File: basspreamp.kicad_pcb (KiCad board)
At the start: 2 copper layers, 62.2 x 44.5 mm, 27 parts, among them P1 INPUT, P2 OUTPUT, P3 Power, Q1 J201, U1 TL072

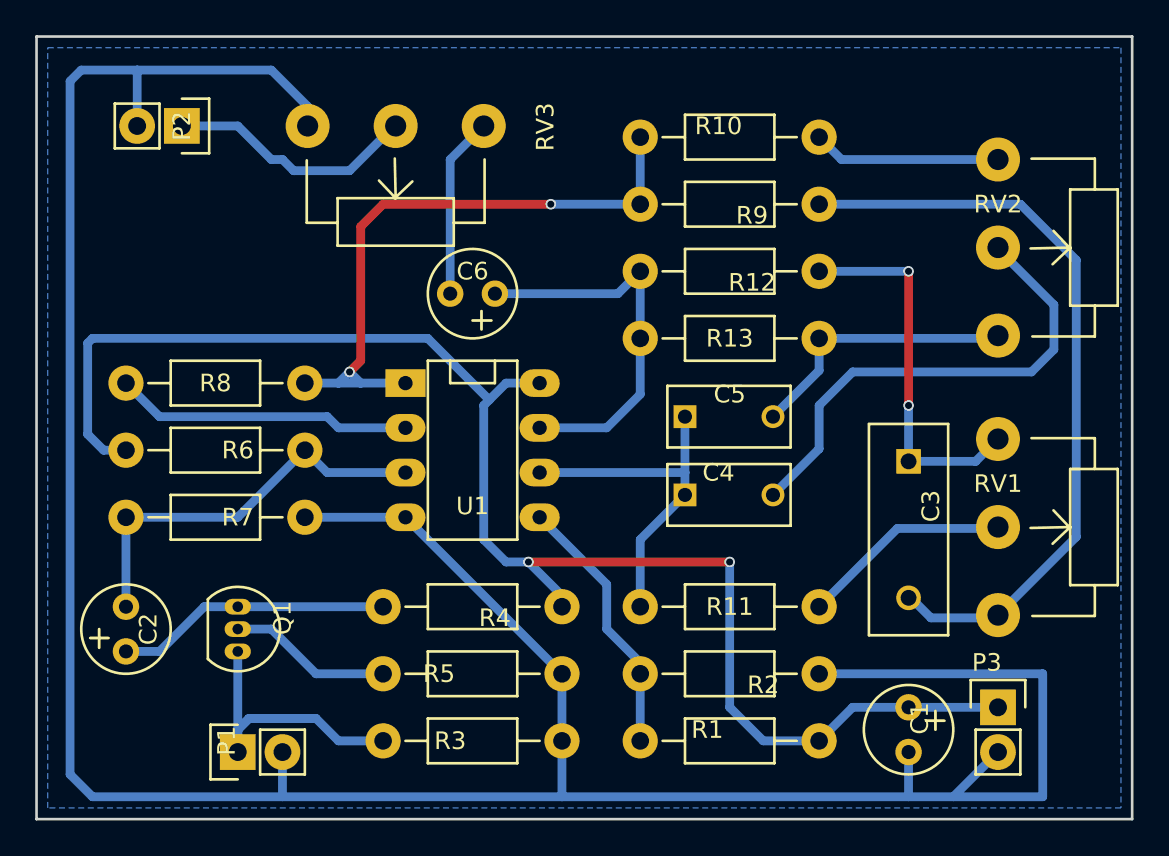
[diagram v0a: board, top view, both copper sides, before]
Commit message: PCB
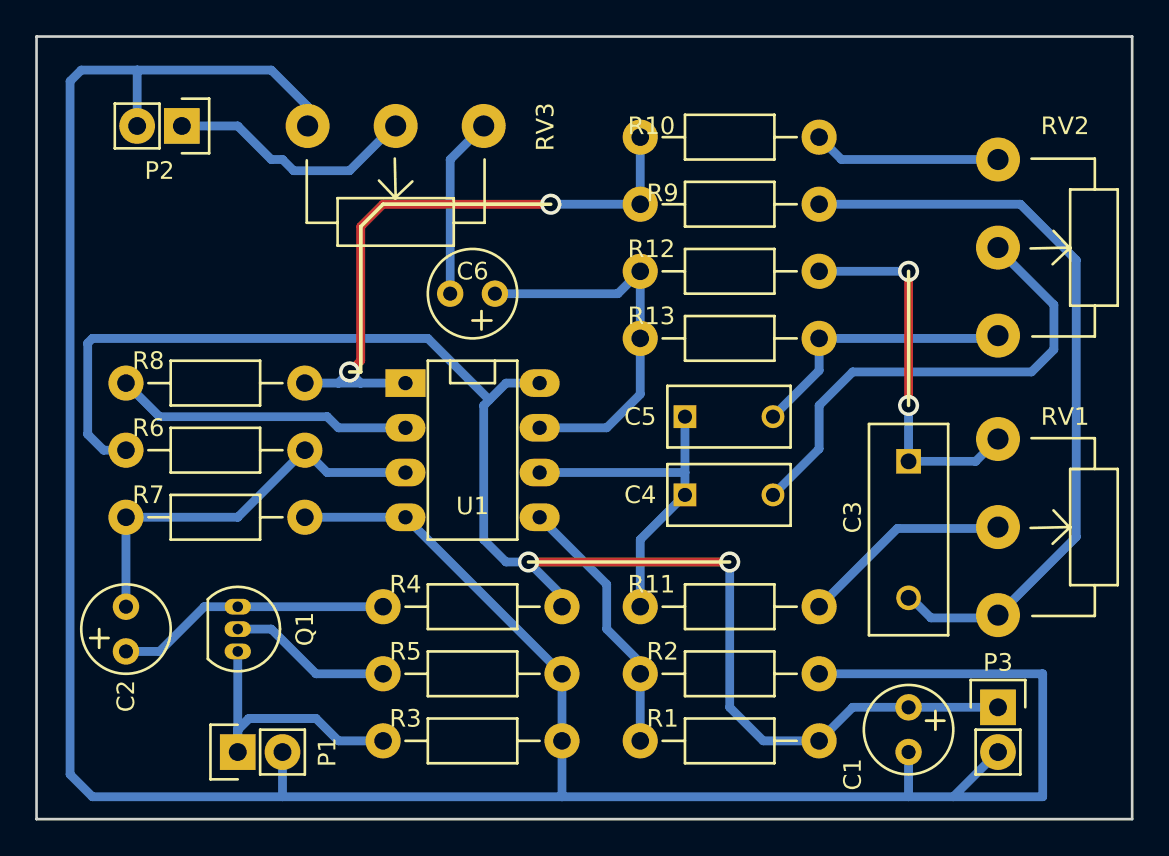
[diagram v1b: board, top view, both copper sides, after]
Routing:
- removed copper zone on B.Cu, net Earth
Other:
- net class Default: via_dia 0.6 -> 1.2; via_drill 0.4 -> 0.8
